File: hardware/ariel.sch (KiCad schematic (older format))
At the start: 20 parts, among them SW1 SW_Push, U1 WeMos_Battery_Shield, U2 WeMos_D1_mini, U3 74HC595, U4 Si7021_breakout

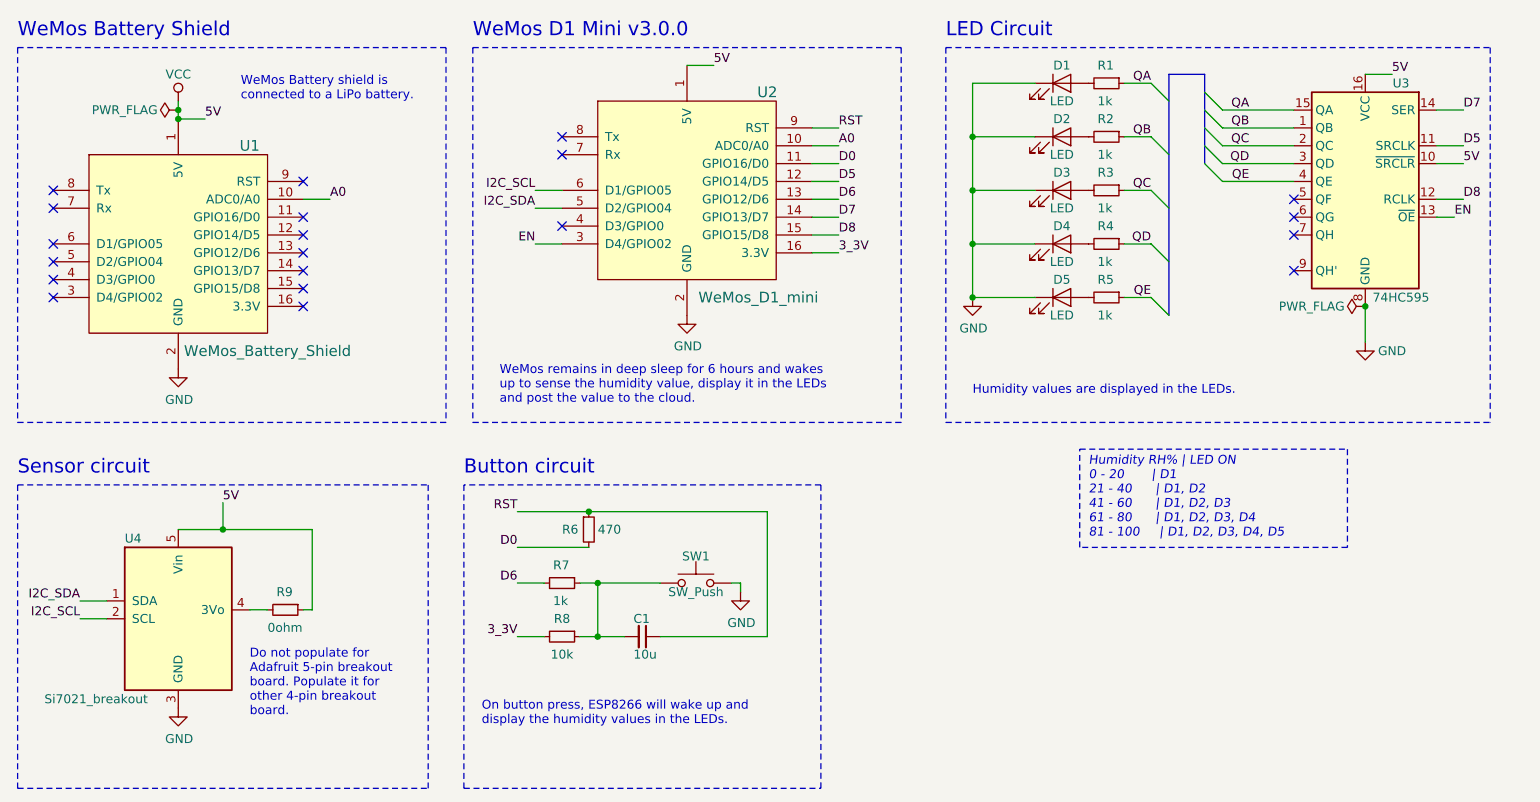
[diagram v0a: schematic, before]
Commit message: Add mechanical pieces
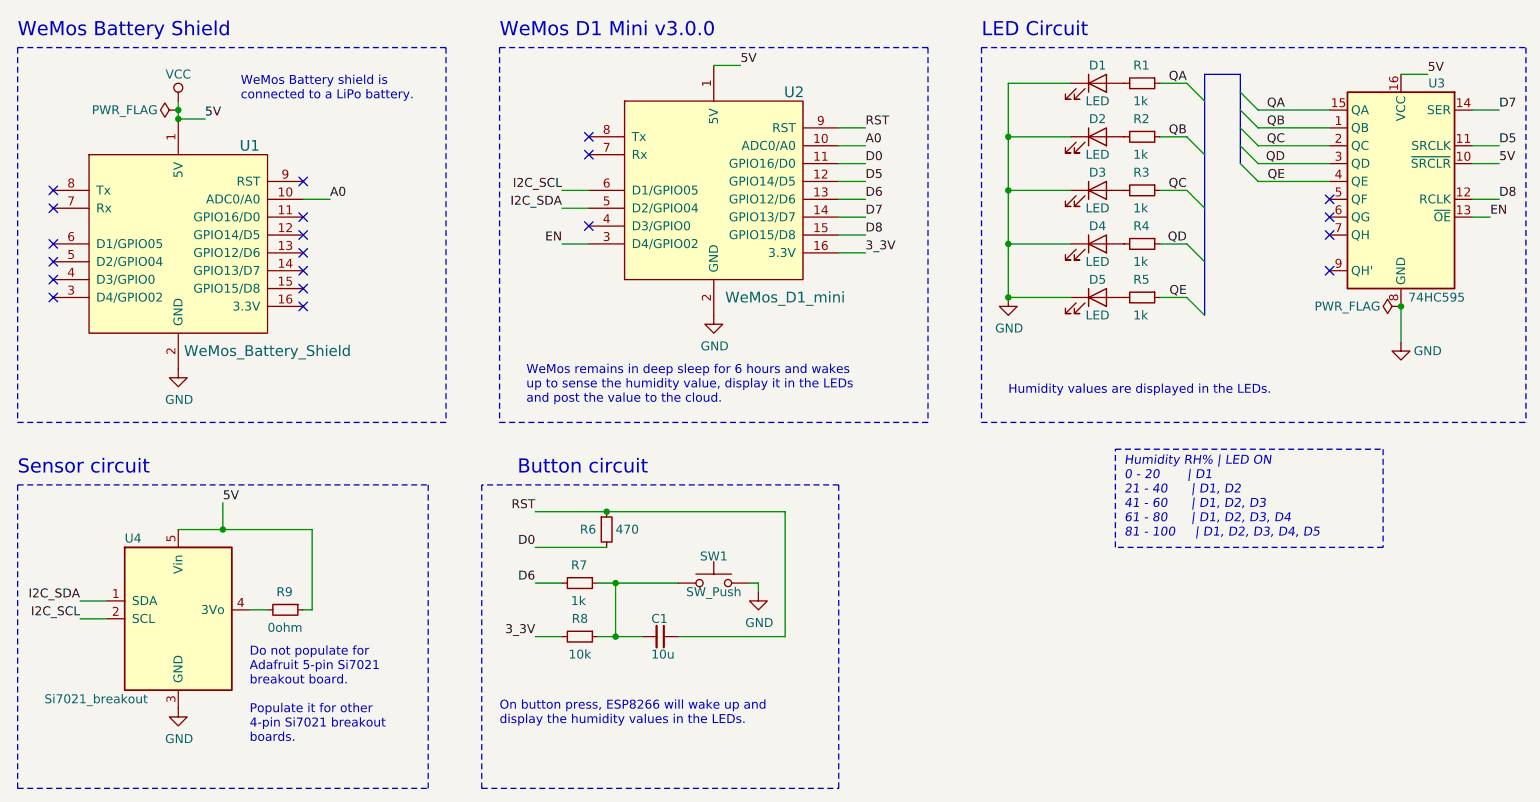
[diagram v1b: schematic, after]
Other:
- note added: "Do not populate for \nAdafruit 5-pin Si7021 \nbreakout board. \n\nPopulate it for other \n4-pin Si7021 breakout \nboards."
- note removed: "Do not populate for \nAdafruit 5-pin breakout \nboard. Populate it for \nother 4-pin breakout \nboard."
- moved on the sheet: C1, D1, D2, D3, D4, D5, R1, R2, R3, R4, R5, R6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
